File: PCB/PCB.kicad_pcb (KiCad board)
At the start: 2 copper layers, 44.7 x 72.6 mm, 23 parts, among them J1 Conn_01x04_Female, J2 Conn_01x05_Female, J3 Screw_Terminal_01x02, J4 Conn_01x03_Female, J5 Conn_01x03_Female, J6 Conn_01x03_Female, J7 Conn_01x03_Female, U1 R-785.0-1.0

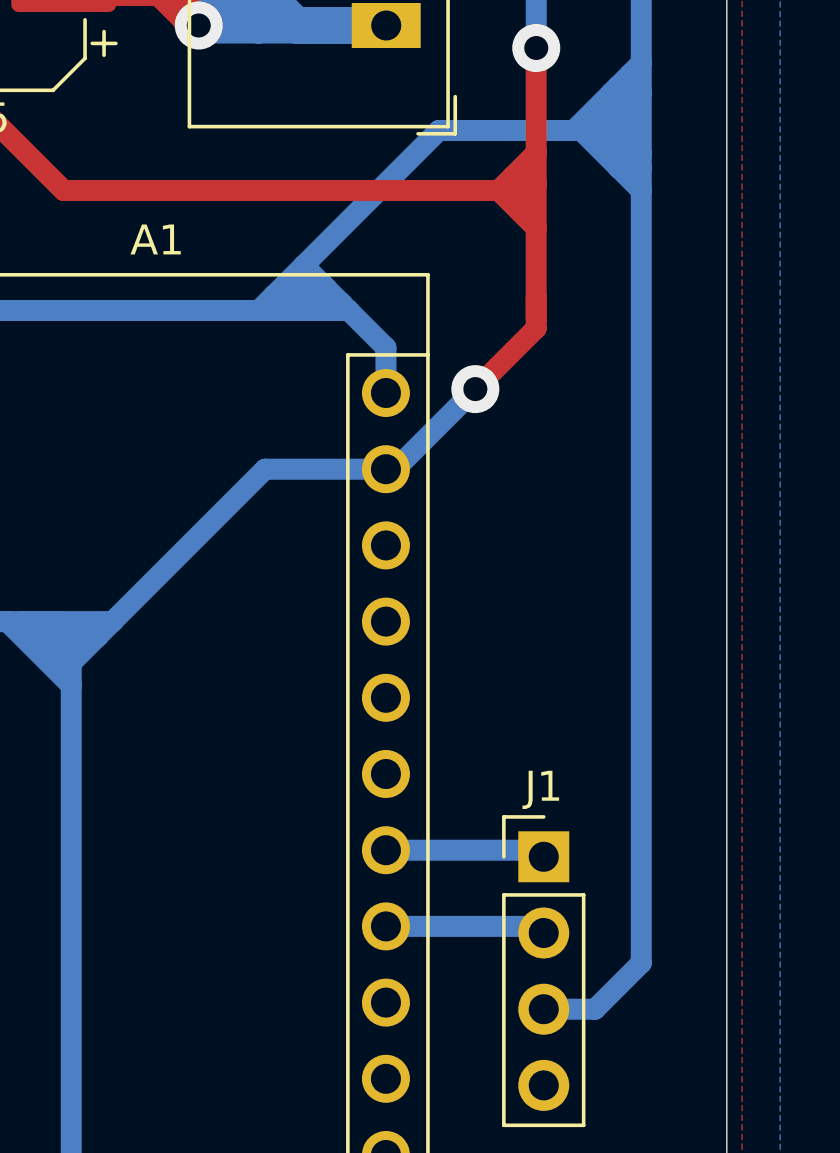
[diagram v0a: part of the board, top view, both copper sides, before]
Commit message: Add files via upload
MàJ
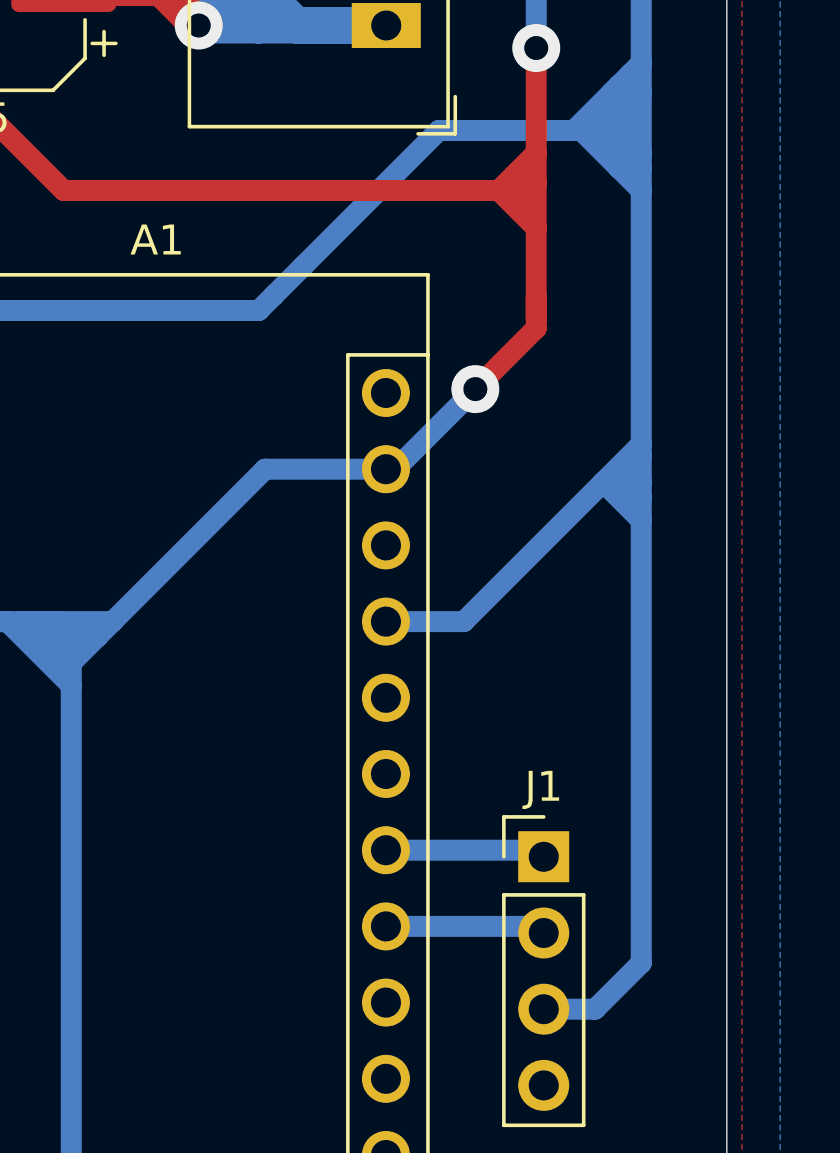
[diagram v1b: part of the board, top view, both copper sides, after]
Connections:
- A1 pad 27: Net-(A1-Pad27) -> +5V
- A1 pad 30: +5V -> Net-(A1-Pad30)
